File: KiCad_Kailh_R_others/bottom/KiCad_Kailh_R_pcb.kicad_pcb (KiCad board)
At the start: 2 copper layers, 138.1 x 100 mm, 0 parts

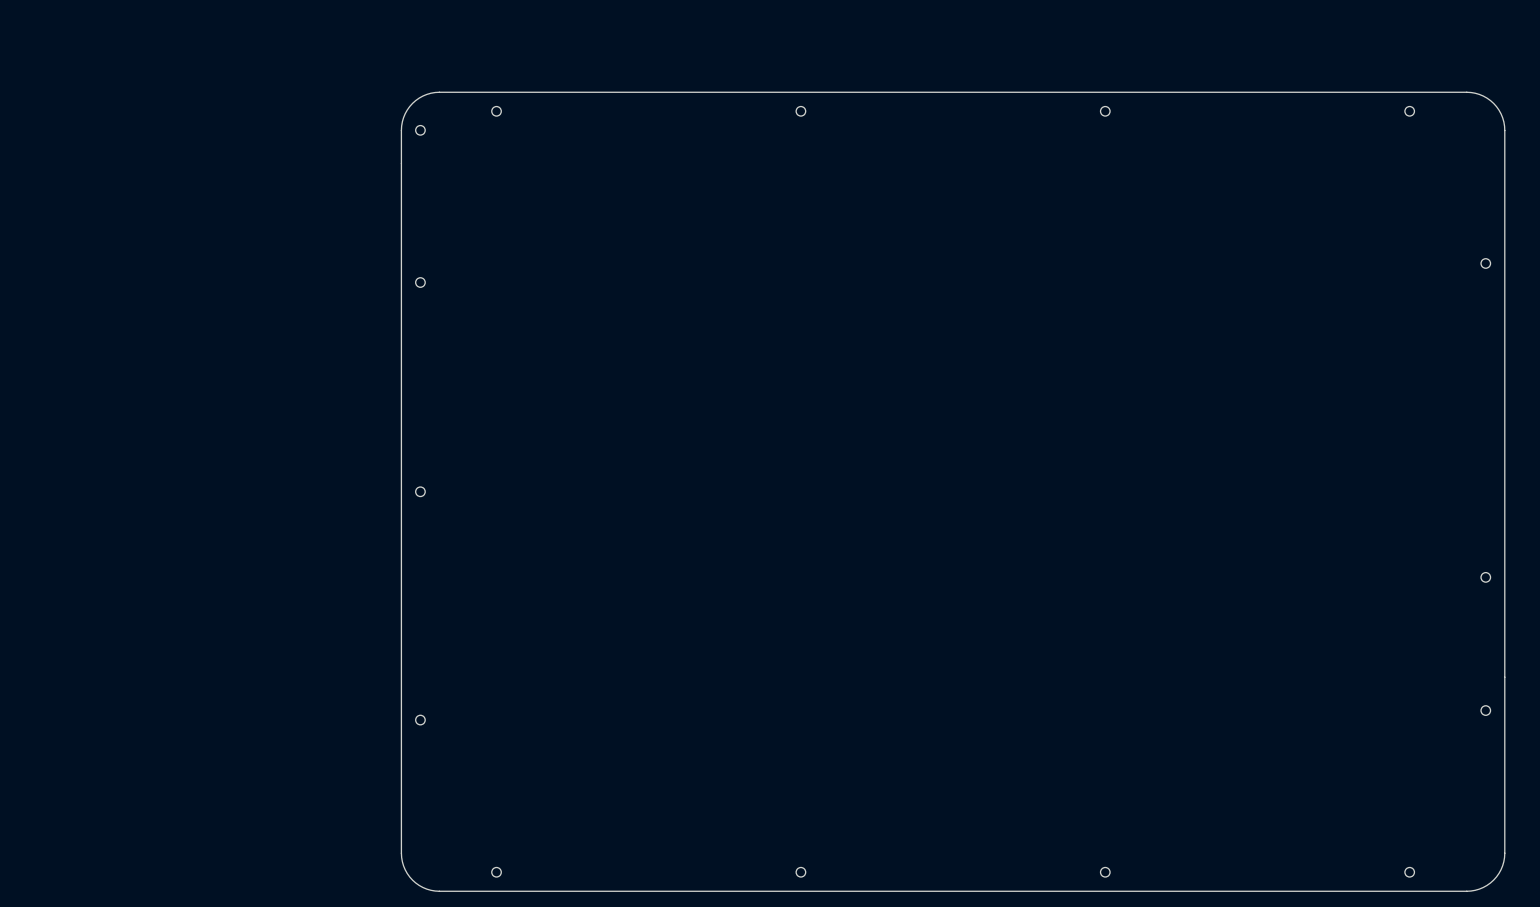
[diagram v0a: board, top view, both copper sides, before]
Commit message: feat: ガワがすべて完成
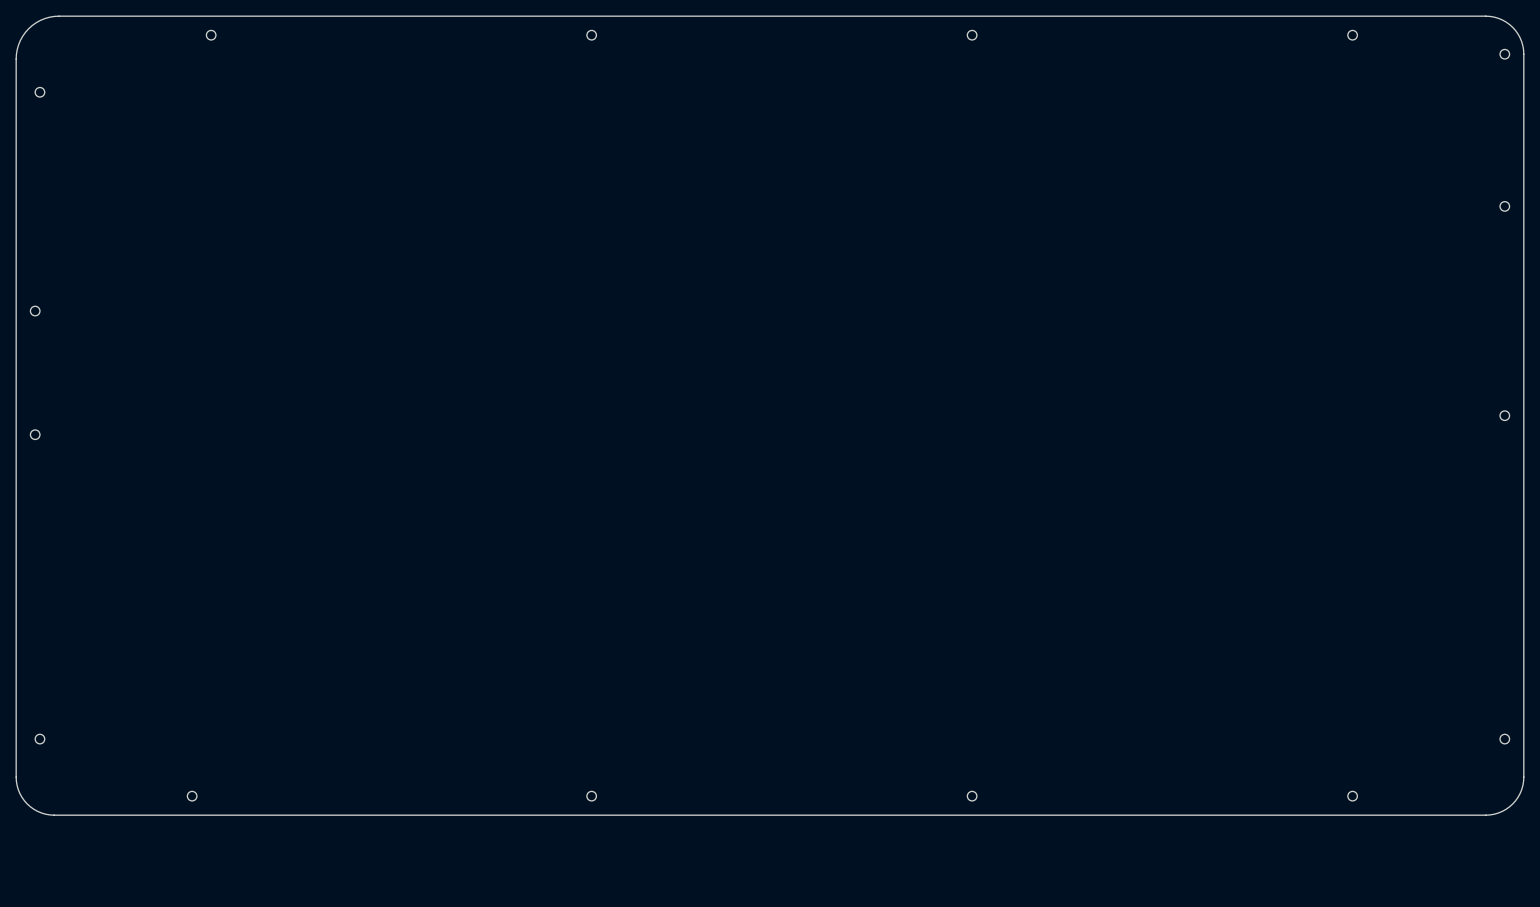
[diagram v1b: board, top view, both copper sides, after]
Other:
- board size 138.1 x 100 mm -> 188.7 x 100 mm
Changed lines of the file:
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@@
 	(net 0 "")
 	(gr_arc
-		(start 80.96253 50.00625)
-		(mid 82.357436 46.638677)
-		(end 85.725 45.24375)
-		(stroke
-			(width 0.05)
-			(type default)
-		)
-		(layer "Edge.Cuts")
-	)
-	(gr_line
-		(start 80.962568 54.173483)
-		(end 80.962501 50.00625)
-		(stroke
-			(width 0.05)
-			(type default)
-		)
-		(layer "Edge.Cuts")
-	)
-	(gr_line
-		(start 80.962568 54.173483)
-		(end 80.9625 140.49372)
-		(stroke
-			(width 0.05)
-			(type default)
-		)
-		(layer "Edge.Cuts")
-	)
-	(gr_circle
-		(center 83.34382 50.006292)
-		(end 83.939133 50.006292)
-		(stroke
-			(width 0.05)
-			(type default)
-		)
-		(fill no)
-		(layer "Edge.Cuts")
-	)
-	(gr_circle
-		(center 83.34382 69.056308)
-		(end 83.939133 69.056308)
-		(stroke
-			(width 0.05)
-			(type default)
-		)
-		(fill no)
-		(layer "Edge.Cuts")
-	)
-	(gr_circle
-		(center 83.34382 95.25008)
-		(end 83.939133 95.25008)
-		(stroke
-			(width 0.05)
-			(type default)
-		)
-		(fill no)
-		(layer "Edge.Cuts")
-	)
-	(gr_circle
-		(center 83.34382 123.825104)
-		(end 83.939133 123.825104)
-		(stroke
-			(width 0.05)
-			(type default)
-		)
-		(fill no)
-		(layer "Edge.Cuts")
-	)
-	(gr_arc
-		(start 85.725 145.25625)
-		(mid 82.357482 143.861303)
-		(end 80.96269 140.49372)
-		(stroke
-			(width 0.05)
-			(type default)
-		)
-		(layer "Edge.Cuts")
-	)
-	(gr_circle
-		(center 92.868828 47.62504)
-		(end 93.464141 47.62504)
-		(stroke
-			(width 0.05)
-			(type default)
-		)
-		(fill no)
-		(layer "Edge.Cuts")
-	)
-	(gr_circle
-		(center 92.868828 142.87512)
-		(end 93.464141 142.87512)
-		(stroke
-			(width 0.05)
-			(type default)
-		)
-		(fill no)
-		(layer "Edge.Cuts")
-	)
-	(gr_circle
-		(center 130.96886 47.62504)
-		(end 131.564173 47.62504)
-		(stroke
-			(width 0.05)
-			(type default)
-		)
-		(fill no)
-		(layer "Edge.Cuts")
-	)
-	(gr_circle
-		(center 130.96886 142.87512)
-		(end 131.564173 142.87512)
-		(stroke
-			(width 0.05)
-			(type default)
-		)
-		(fill no)
-		(layer "Edge.Cuts")
-	)
-	(gr_circle
-		(center 169.068892 47.62504)
-		(end 169.664205 47.62504)
-		(stroke
-			(width 0.05)
-			(type default)
-		)
-		(fill no)
-		(layer "Edge.Cuts")
-	)
-	(gr_circle
-		(center 169.068892 142.87512)
-		(end 169.664205 142.87512)
-		(stroke
-			(width 0.05)
-			(type default)
-		)
-		(fill no)
-		(layer "Edge.Cuts")
-	)
-	(gr_circle
-		(center 207.168924 47.62504)
-		(end 207.764237 47.62504)
-		(stroke
-			(width 0.05)
-			(type default)
-		)
-		(fill no)
-		(layer "Edge.Cuts")
-	)
-	(gr_circle
-		(center 207.168924 142.87512)
-		(end 207.764237 142.87512)
-		(stroke
-			(width 0.05)
-			(type default)
-		)
-		(fill no)
-		(layer "Edge.Cuts")
-	)
-	(gr_line
-		(start 214.3125 45.24375)
-		(end 85.725 45.24375)
-		(stroke
-			(width 0.05)
-			(type default)
-		)
-		(layer "Edge.Cuts")
-	)
-	(gr_arc
-		(start 214.3125 45.24375)
-		(mid 217.687952 46.64633)
-		(end 219.075172 50.028124)
-		(stroke
-			(width 0.05)
-			(type default)
-		)
-		(layer "Edge.Cuts")
-	)
-	(gr_line
-		(start 214.3125 145.2562)
-		(end 85.725 145.25625)
-		(stroke
-			(width 0.05)
-			(type default)
-		)
-		(layer "Edge.Cuts")
-	)
-	(gr_circle
-		(center 216.693932 66.675056)
-		(end 217.289245 66.675056)
-		(stroke
-			(width 0.05)
-			(type default)
-		)
-		(fill no)
-		(layer "Edge.Cuts")
-	)
-	(gr_circle
-		(center 216.693932 105.965714)
-		(end 217.289245 105.965714)
-		(stroke
-			(width 0.05)
-			(type default)
-		)
-		(fill no)
-		(layer "Edge.Cuts")
-	)
-	(gr_circle
-		(center 216.693932 122.634478)
-		(end 217.289245 122.634478)
-		(stroke
-			(width 0.05)
-			(type default)
-		)
-		(fill no)
-		(layer "Edge.Cuts")
-	)
-	(gr_line
-		(start 219.075 50.028123)
-		(end 219.075184 118.467287)
-		(stroke
-			(width 0.05)
-			(type default)
-		)
-		(layer "Edge.Cuts")
-	)
-	(gr_arc
-		(start 219.075 140.49375)
-		(mid 217.680127 143.861359)
-		(end 214.3125 145.256188)
-		(stroke
-			(width 0.05)
-			(type default)
-		)
-		(layer "Edge.Cuts")
-	)
-	(gr_line
-		(start 219.075184 118.467287)
-		(end 219.075 140.49375)
-		(stroke
-			(width 0.05)
+		(start 32.74222 41.076597)
+		(mid 34.311487 37.288052)
+		(end 38.100032 35.718785)
+		(stroke
+			(width 0.05)
+			(type default)
+		)
+		(layer "Edge.Cuts")
+	)
+	(gr_line
+		(start 32.74222 41.0766)
+		(end 32.742215 130.96886)
+		(stroke
+			(width 0.05)
+			(type default)
+		)
+		(layer "Edge.Cuts")
+	)
+	(gr_circle
+		(center 35.123467 72.628186)
+		(end 35.71878 72.628186)
+		(stroke
+			(width 0.05)
+			(type default)
+		)
+		(fill no)
+		(layer "Edge.Cuts")
+	)
+	(gr_circle
+		(center 35.123467 88.106324)
+		(end 35.71878 88.106324)
+		(stroke
+			(width 0.05)
+			(type default)
+		)
+		(fill no)
+		(layer "Edge.Cuts")
+	)
+	(gr_circle
+		(center 35.71878 45.243788)
+		(end 36.314093 45.243788)
+		(stroke
+			(width 0.05)
+			(type default)
+		)
+		(fill no)
+		(layer "Edge.Cuts")
+	)
+	(gr_circle
+		(center 35.71878 126.206356)
+		(end 36.314093 126.206356)
+		(stroke
+			(width 0.05)
+			(type default)
+		)
+		(fill no)
+		(layer "Edge.Cuts")
+	)
+	(gr_arc
+		(start 37.5047 135.731364)
+		(mid 34.137113 134.336452)
+		(end 32.742215 130.96886)
+		(stroke
+			(width 0.05)
+			(type default)
+		)
+		(layer "Edge.Cuts")
+	)
+	(gr_line
+		(start 38.100032 35.718785)
+		(end 216.69375 35.71878)
+		(stroke
+			(width 0.05)
+			(type default)
+		)
+		(layer "Edge.Cuts")
+	)
+	(gr_circle
+		(center 54.768796 133.350112)
+		(end 55.364109 133.350112)
+		(stroke
+			(width 0.05)
+			(type default)
+		)
+		(fill no)
+		(layer "Edge.Cuts")
+	)
+	(gr_circle
+		(center 57.150048 38.100032)
+		(end 57.745361 38.100032)
+		(stroke
+			(width 0.05)
+			(type default)
+		)
+		(fill no)
+		(layer "Edge.Cuts")
+	)
+	(gr_circle
+		(center 104.775088 38.100032)
+		(end 105.370401 38.100032)
+		(stroke
+			(width 0.05)
+			(type default)
+		)
+		(fill no)
+		(layer "Edge.Cuts")
+	)
+	(gr_circle
+		(center 104.775088 133.350112)
+		(end 105.370401 133.350112)
+		(stroke
+			(width 0.05)
+			(type default)
+		)
+		(fill no)
+		(layer "Edge.Cuts")
+	)
+	(gr_circle
+		(center 152.400128 38.100032)
+		(end 152.995441 38.100032)
+		(stroke
+			(width 0.05)
+			(type default)
+		)
+		(fill no)
+		(layer "Edge.Cuts")
+	)
+	(gr_circle
+		(center 152.400128 133.350112)
+		(end 152.995441 133.350112)
+		(stroke
+			(width 0.05)
+			(type default)
+		)
+		(fill no)
+		(layer "Edge.Cuts")
+	)
+	(gr_circle
+		(center 200.025168 38.100032)
+		(end 200.620481 38.100032)
+		(stroke
+			(width 0.05)
+			(type default)
+		)
+		(fill no)
+		(layer "Edge.Cuts")
+	)
+	(gr_circle
+		(center 200.025168 133.350112)
+		(end 200.620481 133.350112)
+		(stroke
+			(width 0.05)
+			(type default)
+		)
+		(fill no)
+		(layer "Edge.Cuts")
+	)
+	(gr_arc
+		(start 216.69375 35.71878)
+		(mid 220.061467 37.113621)
+		(end 221.456436 40.481284)
+		(stroke
+			(width 0.05)
+			(type default)
+		)
+		(layer "Edge.Cuts")
+	)
+	(gr_line
+		(start 216.693932 135.731364)
+		(end 37.50472 135.731364)
+		(stroke
+			(width 0.05)
+			(type default)
+		)
+		(layer "Edge.Cuts")
+	)
+	(gr_circle
+		(center 219.075184 40.481284)
+		(end 219.670497 40.481284)
+		(stroke
+			(width 0.05)
+			(type default)
+		)
+		(fill no)
+		(layer "Edge.Cuts")
+	)
+	(gr_circle
+		(center 219.075184 59.5313)
+		(end 219.670497 59.5313)
+		(stroke
+			(width 0.05)
+			(type default)
+		)
+		(fill no)
+		(layer "Edge.Cuts")
+	)
+	(gr_circle
+		(center 219.075184 85.725072)
+		(end 219.670497 85.725072)
+		(stroke
+			(width 0.05)
+			(type default)
+		)
+		(fill no)
+		(layer "Edge.Cuts")
+	)
+	(gr_circle
+		(center 219.075184 126.206356)
+		(end 219.670497 126.206356)
+		(stroke
+			(width 0.05)
+			(type default)
+		)
+		(fill no)
+		(layer "Edge.Cuts")
+	)
+	(gr_line
+		(start 221.456436 40.481284)
+		(end 221.456436 130.96886)
+		(stroke
+			(width 0.05)
+			(type default)
+		)
+		(layer "Edge.Cuts")
+	)
+	(gr_arc
+		(start 221.456436 130.96886)
+		(mid 220.061531 134.336459)
+		(end 216.693932 135.731364)
+		(stroke
+			(width 0.05)
